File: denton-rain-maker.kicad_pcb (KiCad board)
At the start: 2 copper layers, 75 x 75 mm, 68 parts, among them J1 Conn_01x06, J2 MOV, J3 SEED C3, Q4 BT136S-800E, Q5 BT136S-800E, Q6 BT136S-800E, Q7 BT136S-800E, U1 LMR38020FSDDAR, U2 TLV1117-33, U4 MOC3063M, U6 MOC3063M, U7 MOC3063M, U8 MOC3063M

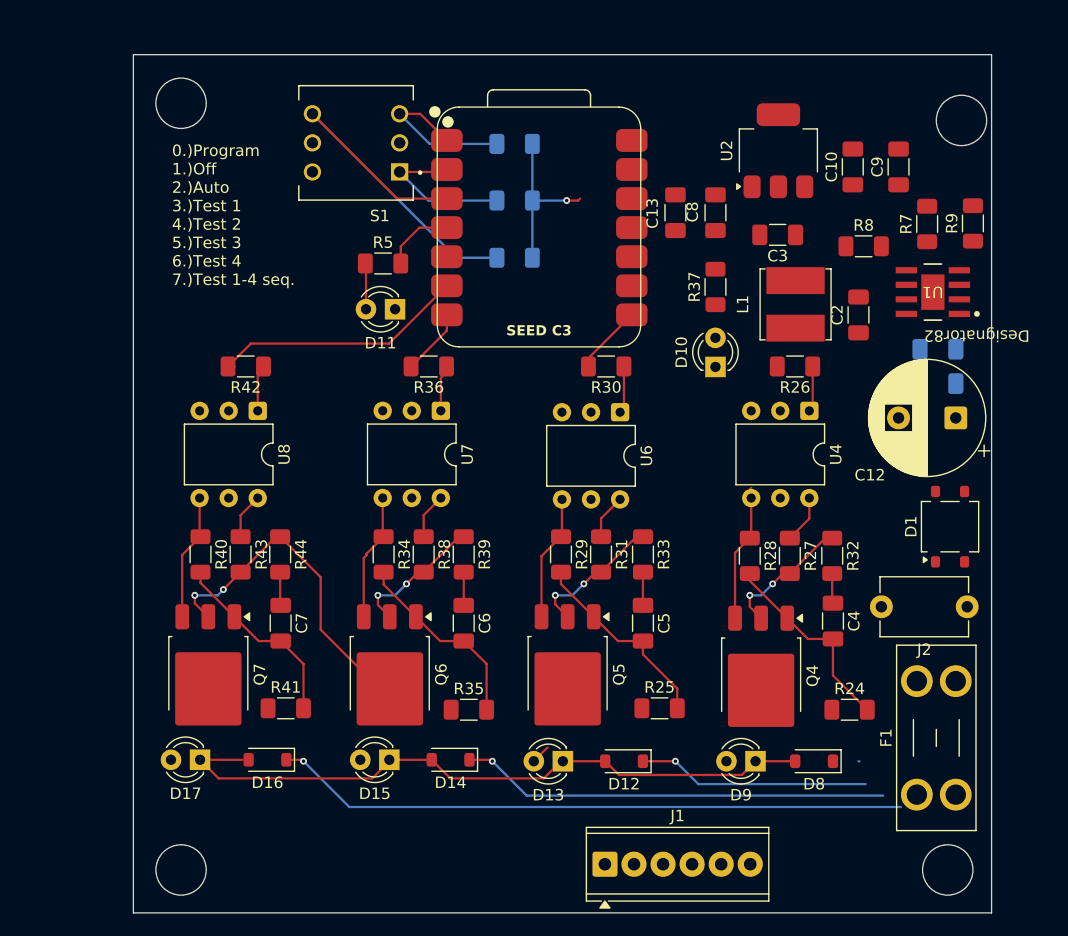
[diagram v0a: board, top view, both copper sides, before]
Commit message: new pwr supply
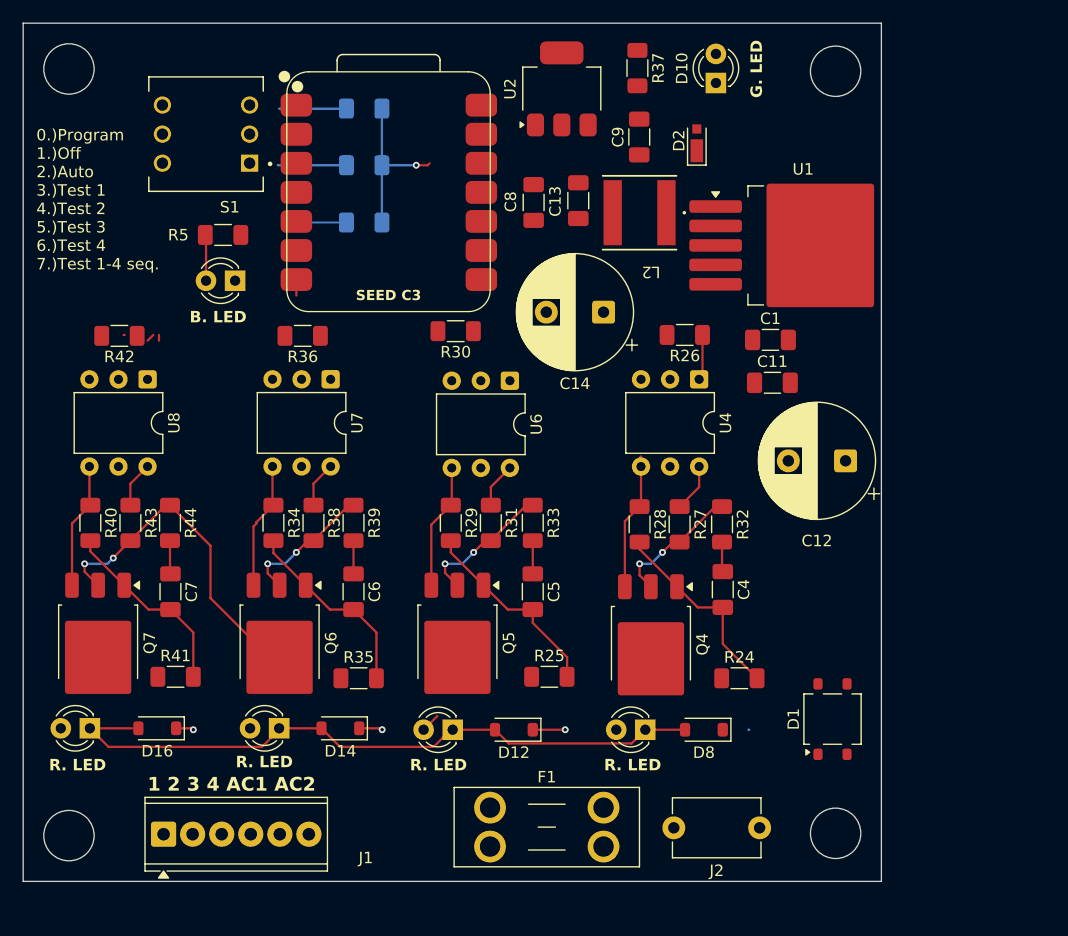
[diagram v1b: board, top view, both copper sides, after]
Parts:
- removed C10, C3: 22uF, Capacitor_SMD:C_1206_3216Metric_Pad1.33x1.80mm_HandSolder
- removed C2: 2.2nF, Capacitor_SMD:C_1206_3216Metric_Pad1.33x1.80mm_HandSolder
- removed L1: 47uH, Inductor_SMD:L_Bourns_SRN6045TA
- removed R7: 24.9k, Resistor_SMD:R_1206_3216Metric_Pad1.30x1.75mm_HandSolder
- removed R8: 100k, Resistor_SMD:R_1206_3216Metric_Pad1.30x1.75mm_HandSolder
- removed R9: 250k, Resistor_SMD:R_1206_3216Metric_Pad1.30x1.75mm_HandSolder
- added C14: 220uF, Capacitor_THT:CP_Radial_D10.0mm_P5.00mm, F.Cu at (161.7, 74.3)
- added D2: D_Schottky_Small, Diode_SMD:D_MicroSMP_LargeCathode, F.Cu at (169.9, 59.3)
- added L2: NRS6028T330MMGJ, inductor:IND_TAIYO_NRS6028_TAY, F.Cu at (164.9, 65.6)
- C1, C11: moved to F.Cu
- U1: value LMR38020FSDDAR -> LM2596S-5; footprint footprints:DDA0008E-IPC_C -> Package_TO_SOT_SMD:TO-263-5_TabPin3
- moved J1 38.7 mm to (123.3, 119.9)
- moved F1 37.3 mm to (151.8, 117.6), turned to 0 degrees
- moved J2 26.5 mm to (175.4, 119.3)
- moved D10 24.8 mm to (171.5, 54.2)
- moved C9 22.8 mm to (164.8, 58.9)
- moved R37 20.3 mm to (164.7, 52.9), turned to -90 degrees
- moved D1 19.7 mm to (181.7, 109.8)
- moved U2 19.7 mm to (158.1, 54.7)
- moved C8 15.9 mm to (155.6, 64.7)
- moved C1 14.7 mm to (176.3, 76.7), turned to 0 degrees
- moved C11 14.5 mm to (176.5, 80.4), turned to 0 degrees
- moved D11 14.2 mm to (129.5, 71.5)
- moved R5 14.2 mm to (128.5, 67.5)
- moved J3 13.5 mm to (142.9, 63.7)
- moved R13 13.5 mm to (140.8, 66.4)
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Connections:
- C9 pad 1: Net-(U2-VI) -> Net-(U1-FB)
- R37 pad 2: Net-(U2-VI) -> Net-(U1-FB)
- U1 pad 1: GND -> Net-(D1-+)
- U1 pad 2: Net-(D1-+) -> Net-(D2-K)
- U1 pad 3: Net-(D1-+) -> GND
- U1 pad 4: Net-(U1-RT_SYNC) -> Net-(U1-FB)
- U1 pad 5: Net-(U1-FB) -> GND
- U2 pad 3: Net-(U2-VI) -> Net-(U1-FB)
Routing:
- net Net-(D16-K): track 72.2 -> 18.3 mm
- net Net-(D14-K): track 54.9 -> 19.5 mm
- net Net-(J3-Pin_6-Pad4): track 36.1 -> 3.54 mm
- net Net-(J3-Pin_3-Pad7): track 22.1 -> 0.10 mm
- net Net-(D12-K): track 37.8 -> 20.4 mm
- net Net-(J3-Pin_8): track 14.7 -> 5.87 mm
- net Net-(J3-Pin_7-Pad3): track 13.7 -> 6.30 mm
- net Net-(J3-Pin_5-Pad5): track 6.20 -> 0.00 mm
- net Net-(J3-Pin_7-Pad20): track 6.08 -> 0.00 mm
- net Net-(J3-Pin_2-Pad21): track 5.80 -> 1.39 mm
- net Net-(R36-Pad1): track 4.08 -> 0.00 mm
- net Net-(R42-Pad1): track 5.29 -> 1.91 mm
- net Net-(R30-Pad1): track 4.14 -> 1.19 mm
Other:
- outline, holes or cut-outs redrawn
- board text added: "1 2 3 4 AC1 AC2"
- board text added: "B. LED"
- board text added: "G. LED"
- board text added: "R. LED"
